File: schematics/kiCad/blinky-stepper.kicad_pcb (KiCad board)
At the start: 2 copper layers, 59 x 53 mm, 13 parts, among them J1 PJ-102A, M3 MountingHole_3.2mm_M3, U1 Teensy-LC, U2 HC06

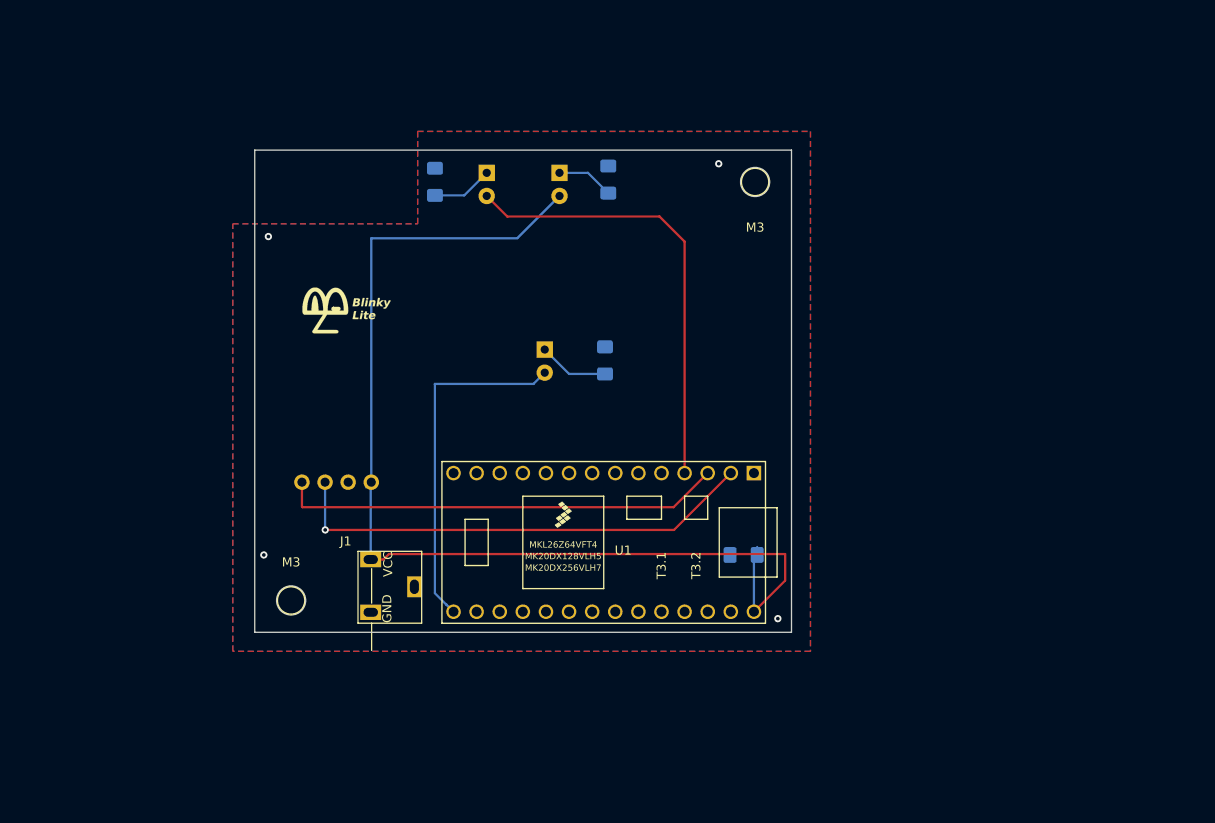
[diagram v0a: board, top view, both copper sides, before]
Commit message: pcb finished
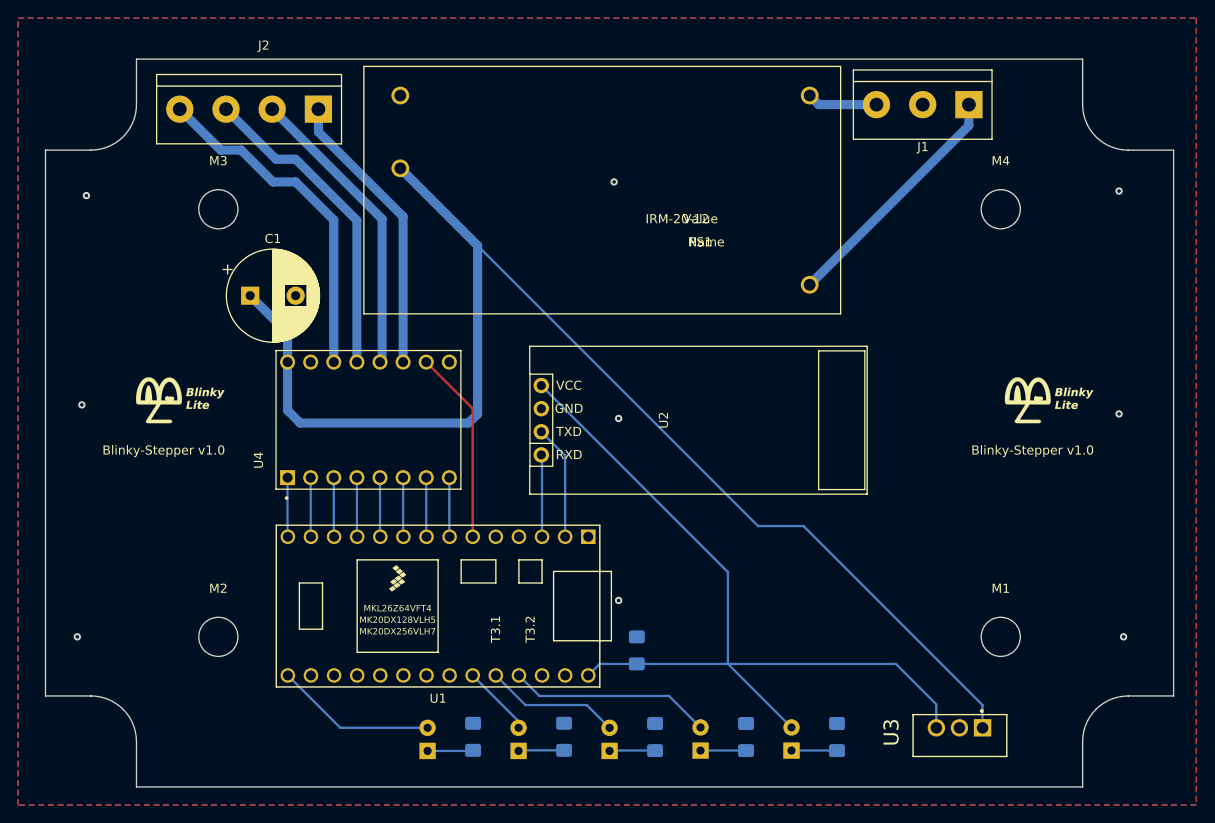
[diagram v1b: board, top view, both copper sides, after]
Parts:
- removed the G*** at (121.3, 87.6)
- removed the M3 at (115.0, 119.5)
- removed the M3 at (166.0, 73.5)
- added C2: 1uF, Capacitor_SMD:C_1206_3216Metric_Pad1.42x1.75mm_HandSolder, B.Cu at (153.0, 125.0)
- added D4: LED, LED_THT:LED_D5.0mm, B.Cu at (150.0, 136.0)
- added D5: LED, LED_THT:LED_D5.0mm, B.Cu at (140.0, 136.0)
- added G***: LOGO, dmcginnis427Footprints:blinkyLiteLogo, F.Cu at (103.0, 97.5)
- added G***: LOGO, dmcginnis427Footprints:blinkyLiteLogo, F.Cu at (198.5, 97.5)
- added J2: Screw_Terminal_01x04, TerminalBlock:TerminalBlock_bornier-4_P5.08mm, F.Cu at (118.0, 65.5)
- added M1: MountingHole_4.3mm_M4, MountingHole:MountingHole_4.3mm_M4, F.Cu at (193.0, 123.5)
- added M2: MountingHole_4.3mm_M4, MountingHole:MountingHole_4.3mm_M4, F.Cu at (107.0, 123.5)
- added M3: MountingHole_4.3mm_M4, MountingHole:MountingHole_4.3mm_M4, F.Cu at (107.0, 76.5)
- added M4: MountingHole_4.3mm_M4, MountingHole:MountingHole_4.3mm_M4, F.Cu at (193.0, 76.5)
- added PS1: IRM-20-12, IRM-20-12:IRM-20-12, F.Cu at (149.2, 74.4)
- added R4: 220, Resistor_SMD:R_1206_3216Metric_Pad1.42x1.75mm_HandSolder, B.Cu at (155.0, 134.5)
- added R5: 220, Resistor_SMD:R_1206_3216Metric_Pad1.42x1.75mm_HandSolder, B.Cu at (145.0, 134.5)
- added U3: L7805ABV, L7805ABV:TO254P460X1020X1945-3P, F.Cu at (188.5, 133.5)
- added U4: DRV8825_STEPPER_MOTOR_DRIVER_CARRIER, DRV8825:IC_DRV8825_STEPPER_MOTOR_DRIVER_CARRIER, F.Cu at (123.5, 99.7)
- C1: value 1uF -> 100uF; footprint Capacitor_SMD:C_1206_3216Metric_Pad1.42x1.75mm_HandSolder -> Capacitor_THT:CP_Radial_D10.0mm_P5.00mm; moved to F.Cu
- J1: value PJ-102A -> Screw_Terminal_01x03; footprint dmcginnis427:DC21Jack -> TerminalBlock:TerminalBlock_bornier-3_P5.08mm
- U2: footprint dmcginnis427:HC06 -> dmcginnis427Footprints:HC06; moved to F.Cu
- moved J1 82.6 mm to (189.5, 65.0), turned to 180 degrees
- moved D1 68.4 mm to (170.0, 136.0), turned to 90 degrees
- moved R1 66.2 mm to (175.0, 134.5)
- moved D2 63.9 mm to (130.0, 136.0), turned to 90 degrees
- moved C1 61.3 mm to (110.5, 86.0)
- moved R2 61.1 mm to (135.0, 134.5)
- moved D3 47.3 mm to (160.0, 136.0), turned to 90 degrees
- moved R3 44.2 mm to (165.0, 134.5)
- moved U2 23.5 mm to (142.5, 99.7), turned to 90 degrees
- moved U1 19.5 mm to (131.2, 120.1)
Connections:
- C1 pad 1: GND -> +12V
- C1 pad 2: +5V -> GND
- J1 pad 1: +5V -> Net-(J1-Pad1)
- J1 pad 3: GND -> Net-(J1-Pad3)
- U1 pad 20: Net-(D3-Pad2) -> Net-(D2-Pad2)
- U1 pad 30: Net-(U1-Pad30) -> Net-(D3-Pad2)
- U1 pad 4: Net-(D2-Pad2) -> Net-(U1-Pad4)
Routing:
- net +12V: track 0.00 -> 145.6 mm
- net Net-(U1-Pad3): track 48.9 -> 9.03 mm
- net Net-(U1-Pad2): track 52.4 -> 12.6 mm, vias 1 -> 0
- net Net-(J2-Pad4): track 0.00 -> 37.6 mm
- net Net-(J2-Pad3): track 0.00 -> 35.0 mm
- net Net-(J2-Pad2): track 0.00 -> 32.9 mm
- net Net-(J2-Pad1): track 0.00 -> 31.7 mm
- net Net-(D2-Pad2): track 49.3 -> 17.7 mm
- net +5V: track 119.8 -> 92.2 mm
- net Net-(J1-Pad1): track 0.00 -> 27.0 mm
- net Net-(U1-Pad6): track 0.00 -> 21.3 mm
- net Net-(D3-Pad2): track 38.5 -> 22.3 mm
- net Net-(D4-Pad2): track 0.00 -> 14.9 mm
- net Net-(D5-Pad2): track 0.00 -> 7.85 mm
- net Net-(J1-Pad3): track 0.00 -> 7.75 mm
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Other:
- board size 59 x 53 mm -> 124 x 80 mm
- board text added: "Blinky-Stepper v1.0"
